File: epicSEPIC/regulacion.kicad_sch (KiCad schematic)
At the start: 13 parts, among them U3 LM7815, U4 LM7805

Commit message: Agregar datasheets
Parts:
- C6, C8: Part Number (none) -> C0603C224M1RACTU
- C7, C9: Part Number (none) -> C0603C104M1RACTU
- U3: Part Number (none) -> LM7815
- U4: Part Number (none) -> LM7805
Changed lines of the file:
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@@
 			)
 		)
-		(property "Datasheet" "~"
+		(property "Datasheet" "https://content.kemet.com/datasheets/KEM_C1002_X7R_SMD.pdf"
 			(at 66.04 33.02 0)
 			(effects
@@
 		)
 		(property "Description" "Unpolarized capacitor"
+			(at 66.04 33.02 0)
+			(effects
+				(font
+					(size 1.27 1.27)
+				)
+				(hide yes)
+			)
+		)
+		(property "Part Number" "C0603C224M1RACTU"
 			(at 66.04 33.02 0)
 			(effects
@@
 			)
 		)
-		(property "Datasheet" "~"
+		(property "Datasheet" "https://content.kemet.com/datasheets/KEM_C1002_X7R_SMD.pdf"
 			(at 116.84 33.02 0)
 			(effects
@@
 		)
 		(property "Description" "Unpolarized capacitor"
+			(at 116.84 33.02 0)
+			(effects
+				(font
+					(size 1.27 1.27)
+				)
+				(hide yes)
+			)
+		)
+		(property "Part Number" "C0603C104M1RACTU"
 			(at 116.84 33.02 0)
 			(effects
@@
 			)
 		)
-		(property "Datasheet" "~"
+		(property "Datasheet" "https://content.kemet.com/datasheets/KEM_C1002_X7R_SMD.pdf"
 			(at 99.06 33.02 0)
 			(effects
@@
 			)
 		)
+		(property "Part Number" "C0603C224M1RACTU"
+			(at 99.06 33.02 0)
+			(effects
+				(font
+					(size 1.27 1.27)
+				)
+				(hide yes)
+			)
+		)
 		(pin "2"
 		)
@@
 			)
 		)
-		(property "Datasheet" "~"
+		(property "Datasheet" "https://content.kemet.com/datasheets/KEM_C1002_X7R_SMD.pdf"
 			(at 250.19 26.67 0)
 			(effects
@@
 			)
 		)
-		(property "Datasheet" "~"
+		(property "Datasheet" "https://content.kemet.com/datasheets/KEM_C1002_X7R_SMD.pdf"
 			(at 83.82 33.02 0)
 			(effects
@@
 			)
 		)
+		(property "Part Number" "C0603C104M1RACTU"
+			(at 83.82 33.02 0)
+			(effects
+				(font
+					(size 1.27 1.27)
+				)
+				(hide yes)
+			)
+		)
 		(pin "2"
 		)
@@
 			)
 		)
+		(property "Part Number" "LM7815"
+			(at 74.93 27.94 0)
+			(effects
+				(font
+					(size 1.27 1.27)
+				)
+				(hide yes)
+			)
+		)
 		(pin "3"
 		)
@@
 			(at 107.95 27.94 0)
 			(effects
+				(font
+					(size 1.27 1.27)
+				)
+				(hide yes)
+			)
+		)
+		(property "Part Number" "LM7805"
+			(at 107.95 27.94 0)
+			(effects

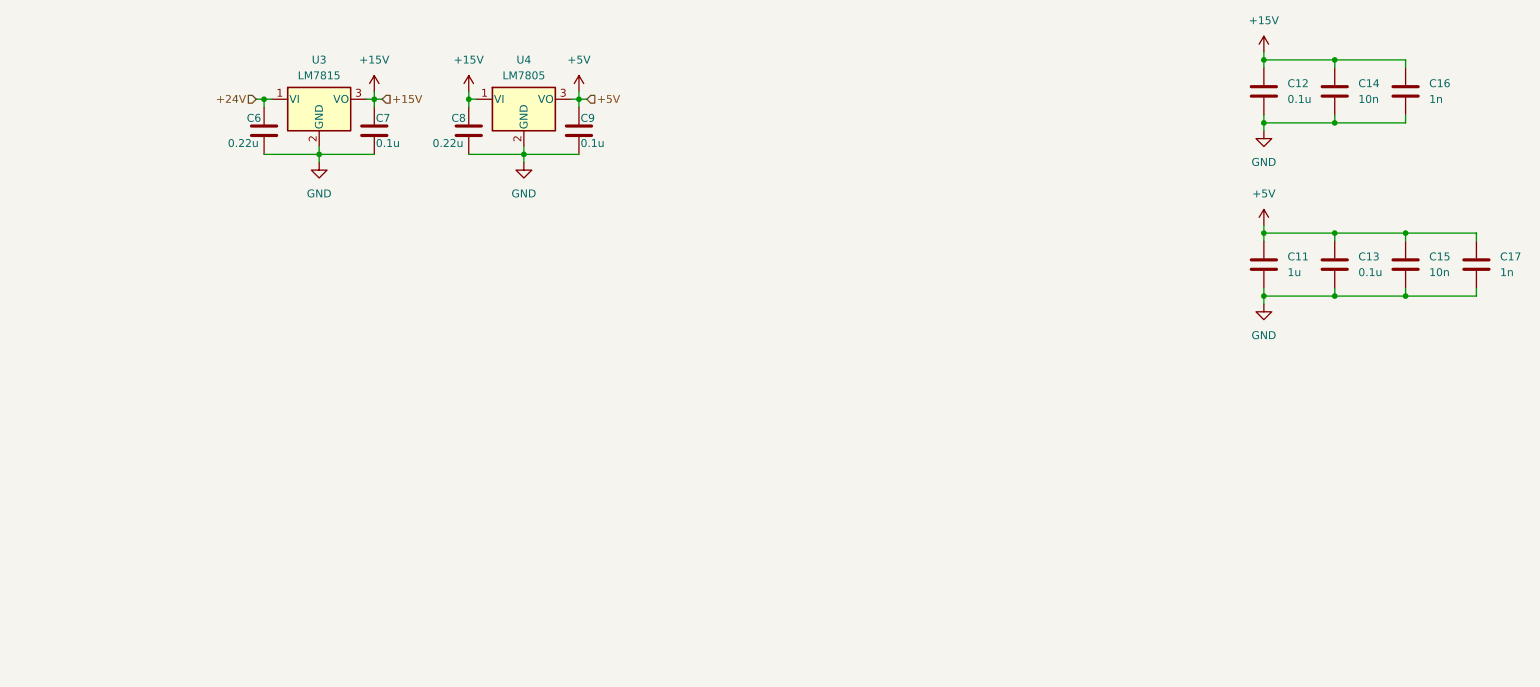
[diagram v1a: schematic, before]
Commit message: PCB Final con reguladores
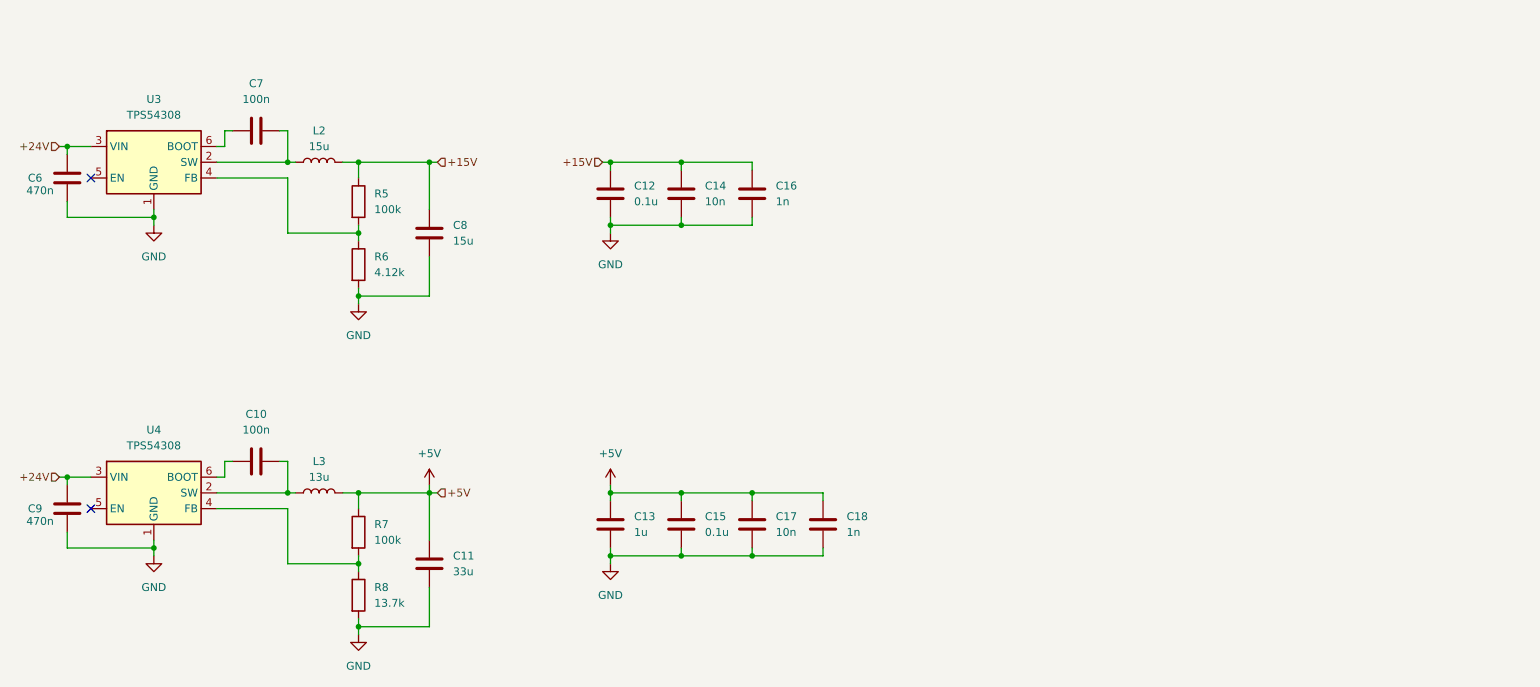
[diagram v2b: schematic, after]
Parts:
- removed U3: LM7815, Package_TO_SOT_SMD:SOT-223-3_TabPin2, symbol Regulator_Linear:LM7815_TO220
- removed U4: LM7805, Package_TO_SOT_SMD:SOT-223-3_TabPin2, symbol Regulator_Linear:LM7805_TO220
- added C10: 100n, Capacitor_SMD:C_0402_1005Metric, symbol Device:C
- added C11: 33u, Capacitor_SMD:C_0805_2012Metric, symbol Device:C
- added L2: 15u, Inductor_SMD_Wurth:L_Wurth_WE-LHMI-7050, symbol Device:L
- added L3: 13u, Inductor_SMD_Wurth:L_Wurth_WE-PDF-1064, symbol Device:L
- added R5, R7: 100k, Resistor_SMD:R_0402_1005Metric, symbol Device:R
- added R6: 4.12k, Resistor_SMD:R_0402_1005Metric, symbol Device:R
- added R8: 13.7k, Resistor_SMD:R_0402_1005Metric, symbol Device:R
- added U3, U4: TPS54308, Package_TO_SOT_SMD:SOT-23-6, symbol Regulator_Switching:TPS54308
- C6: value 0.22u -> 470n; Part Number C0603C224M1RACTU -> CGA3E3X5R1V474K080AB
- C7: value 0.1u -> 100n; footprint Capacitor_SMD:C_0603_1608Metric -> Capacitor_SMD:C_0402_1005Metric; Part Number C0603C104M1RACTU -> C1005X7R1H104K050BB
- C8: value 0.22u -> 15u; footprint Capacitor_SMD:C_0603_1608Metric -> Capacitor_SMD:C_0805_2012Metric; Part Number C0603C224M1RACTU -> C2012X5R1V156M125AC
- C9: value 0.1u -> 470n; Part Number C0603C104M1RACTU -> CGA3E3X5R1V474K080AB
- renumbered C11 to C13, C13 to C15, C15 to C17, C17 to C18
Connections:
- net +15V: now also C8.2, L2.2, R5.1; no longer C7.1, C8.1
- net +24V: now also C9.1, U3.3 (VIN), U4.3 (VIN)
- net +5V: now also C11.2, L3.2, R7.1; no longer C9.1
- net GND: now also C8.1, C11.1, R6.2, R8.2, U3.1 (GND), U4.1 (GND); no longer C7.2, C8.2
- new net: C10.2, L3.1, U4.2 (SW)
- new net: C7.2, L2.1, U3.2 (SW)
- new net: R5.2, R6.1, U3.4 (FB)
- new net: R7.2, R8.1, U4.4 (FB)
- new net: C10.1, U4.6 (BOOT)
- new net: C7.1, U3.6 (BOOT)
- no-connect marks 0 -> 2
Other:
- moved on the sheet: C12, C13, C14, C15, C16, C17, C18

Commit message: Actualizar BOM
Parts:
- C10, C7: Dist (none) -> Mouser; DistPN (none) -> 810-C1005X7R1H104K; Mfg (none) -> TDK; MfgPN (none) -> C1005X7R1H104K050BB; Part Number C1005X7R1H104K050BB -> (none)
- C11: Dist (none) -> Mouser; DistPN (none) -> 810-C2012X5R1A336M125AC; Mfg (none) -> TDK; MfgPN (none) -> C2012X5R1A336M125AC; Part Number C2012X5R1A336M125AC -> (none)
- C12: Dist (none) -> Mouser; DistPN (none) -> 80-C0805C104M4R; Mfg (none) -> Kemet; MfgPN (none) -> C0805C104M4RACTU; Part Number C0805C104M4RACTU -> (none)
- C13: Dist (none) -> Mouser; DistPN (none) -> 80-C0805C105M8R; Mfg (none) -> Kemet; MfgPN (none) -> C0805C105M8RACTU; Part Number C0805C105M8RACTU -> (none)
- C14: Dist (none) -> Mouser; DistPN (none) -> 80-C0603C103M4R; Mfg (none) -> Kemet; MfgPN (none) -> C0603C103M4RACTU; Part Number C0603C103M4RACTU -> (none)
- C15: Dist (none) -> Mouser; DistPN (none) -> 80-C0805C104M8R; Mfg (none) -> Kemet; MfgPN (none) -> C0805C104M8RACTU; Part Number C0805C104M8RACTU -> (none)
- C16: Dist (none) -> Mouser; DistPN (none) -> 80-C0402C102M4R; Mfg (none) -> Kemet; MfgPN (none) -> C0402C102M4RACTU; Part Number C0402C102M4RACTU -> (none)
- C17: Dist (none) -> Mouser; DistPN (none) -> 80-C0603C103M8R; Mfg (none) -> Kemet; MfgPN (none) -> C0603C103M8RACTU; Part Number C0603C103M8RACTU -> (none)
- C18: Dist (none) -> Mouser; DistPN (none) -> 80-C0402C102M8R; Mfg (none) -> Kemet; MfgPN (none) -> C0402C102M8RACTU; Part Number C0402C102M8RACTU -> (none)
- C6, C9: Dist (none) -> Mouser; DistPN (none) -> 810-CGA3E3X5R1V474KB; Mfg (none) -> TDK; MfgPN (none) -> CGA3E3X5R1V474K080AB; Part Number CGA3E3X5R1V474K080AB -> (none)
- C8: Dist (none) -> Mouser; DistPN (none) -> 810-C2012X5R1V156M1C; Mfg (none) -> TDK; MfgPN (none) -> C2012X5R1V156M125AC; Part Number C2012X5R1V156M125AC -> (none)
- L2: Dist (none) -> Mouser; DistPN (none) -> 710-74437349150; Mfg (none) -> Würth Elektronik; MfgPN (none) -> 74437349150; Part Number 74437349150 -> (none)
- L3: Dist (none) -> Mouser; DistPN (none) -> 710-7447798131; Mfg (none) -> Würth Elektronik; MfgPN (none) -> 7447798131; Part Number 7447798131 -> (none)
- R5, R7: Dist (none) -> Mouser; DistPN (none) -> 71-CRCW0402-100K-E3; Mfg (none) -> Vishay; MfgPN (none) -> CRCW0402100KFKED; Part Number CRCW0402100KFKED -> (none)
- R6: Dist (none) -> Mouser; DistPN (none) -> 71-CRCW0402-4.12K-E3; Mfg (none) -> Vishay; MfgPN (none) -> CRCW04024K12FKED; Part Number CRCW04024K12FKED -> (none)
- R8: Dist (none) -> Mouser; DistPN (none) -> 71-CRCW0402-13.7K-E3; Mfg (none) -> Vishay; MfgPN (none) -> CRCW040213K7FKED; Part Number CRCW040213K7FKED -> (none)
- U3, U4: Dist (none) -> Mouser; DistPN (none) -> 595-TPS54308DDCR; Mfg (none) -> Texas Instruments; MfgPN (none) -> TPS54308; Part Number TPS54308 -> (none)
